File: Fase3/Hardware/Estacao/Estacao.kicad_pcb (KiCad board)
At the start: 2 copper layers, 104.1 x 97.8 mm, 33 parts, among them J1 WCM, J2 I2C-1, J3 I2C-2, J4 I2C-3, J5 GPS, J6 Photo Cel, SW1 SW_Wuerth_450301014042, SW2 SW_Wuerth_450301014042, SW3 SW_Wuerth_450301014042, SW4 Config, SW5 Reset

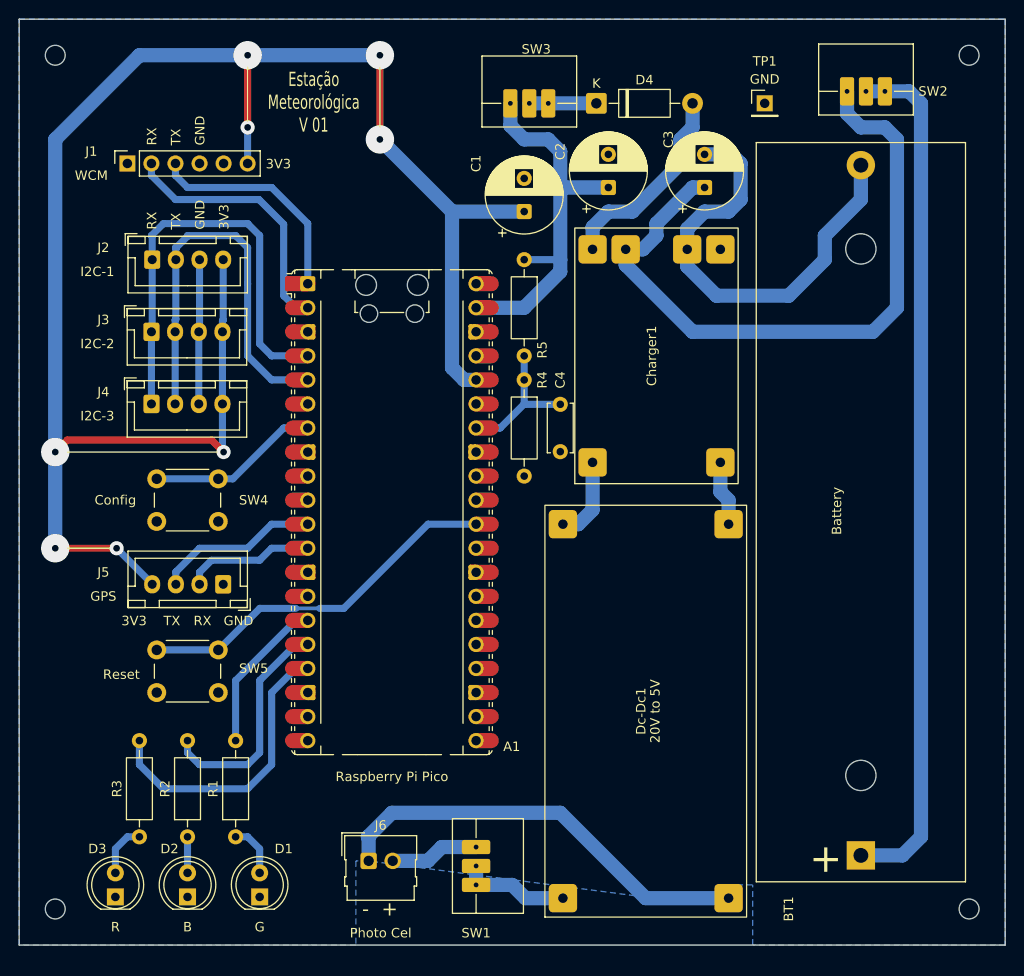
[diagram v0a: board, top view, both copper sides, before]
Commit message: Update PCB V03
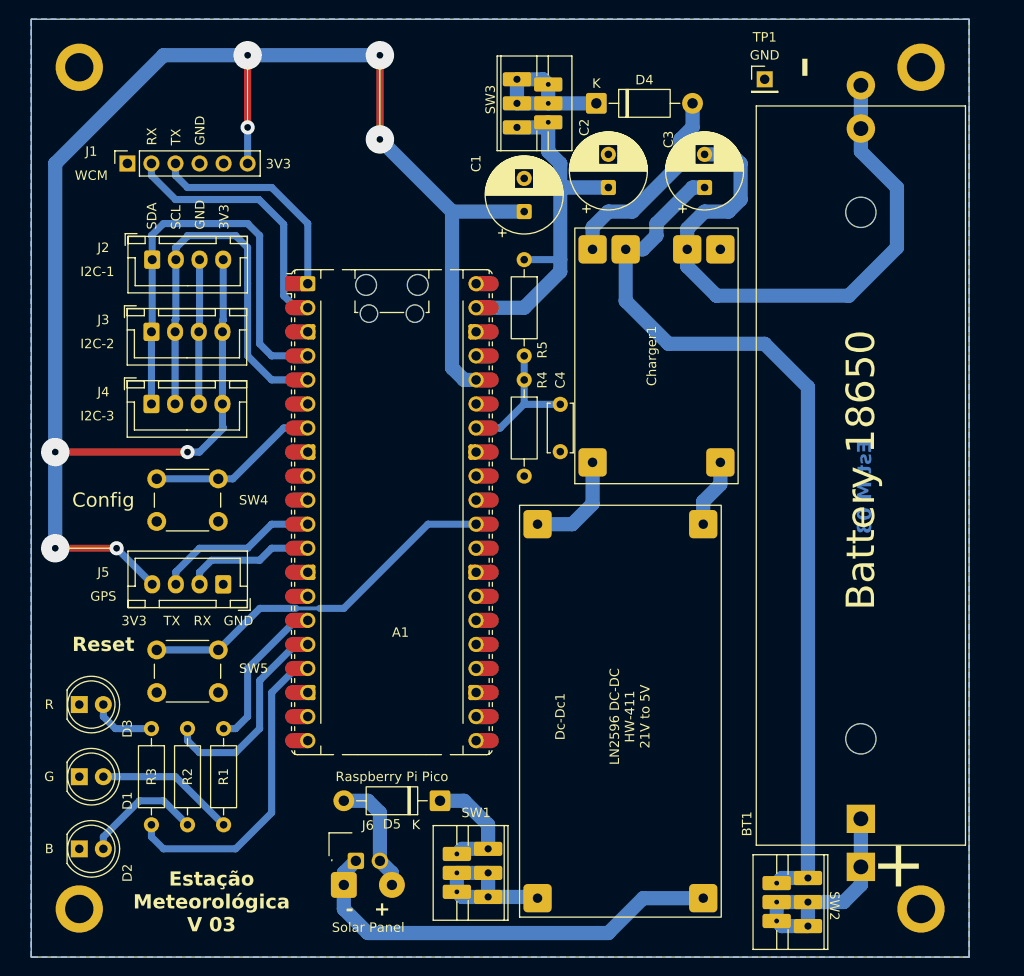
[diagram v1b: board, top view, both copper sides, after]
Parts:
- removed the ? at (194.3, 128.3)
- removed REF** (x3): MountingHole_2.1mm, MountingHole:MountingHole_2.1mm
- added ?: , , F.Cu at (189.2, 39.4)
- added ?: , , F.Cu at (100.3, 39.4)
- added ?: , , F.Cu at (100.3, 128.3)
- added ?: , , F.Cu at (189.2, 128.3)
- added D5: 1N5819, Diode_THT:D_DO-41_SOD81_P10.16mm_Horizontal, F.Cu at (138.4, 116.8)
- BT1: value Battery -> Battery 18650 2000mAh; footprint Battery:BatteryHolder_MPD_BK-18650-PC2 -> PcbLibrary:BatteryHolder_MPD_BK-18650-PC2b
- C3: value C_Polarized -> 100 uF
- C4: value C -> 100n
- Charger1: value ~ -> HW-107
- Dc-Dc1: value 20V to 5V -> LN2596 DC-DC HW-411 21V to 5V
- J6: footprint Connector_Molex:Molex_SL_171971-0002_1x02_P2.54mm_Vertical -> PcbLibrary:Molex_SL_171971-0002_1x02_P2.54mm_Vertical_b
- R1, R2, R3: value R -> 1k
- R4, R5: value R -> 100k
- SW1, SW2, SW3: value SW_Wuerth_450301014042 -> SW_SPDT; footprint PcbLibrary:switch_3p_2mm -> PcbLibrary:switch_3p_2mm_e_2.54mm
- moved SW2 85.8 mm to (177.3, 127.5), turned to -90 degrees
- moved D1 22.9 mm to (100.3, 114.3), turned to 0 degrees
- moved D3 20.7 mm to (100.3, 106.7), turned to 0 degrees
- moved D2 12.5 mm to (100.3, 121.9), turned to 0 degrees
- moved R3 11.5 mm to (108.0, 109.2), turned to -90 degrees
- moved BT1 3.86 mm to (182.9, 118.7)
- moved Dc-Dc1 2.68 mm to (157.5, 107.4)
- moved TP1 2.54 mm to (172.7, 40.6)
- moved R1 1.80 mm to (115.6, 119.4)
- moved SW1 1.46 mm to (143.5, 124.5)
- moved J6 1.35 mm to (129.5, 123.2)
- moved SW3 1.30 mm to (146.6, 43.2), turned to 90 degrees
- moved R2 1.27 mm to (111.8, 119.4)
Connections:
- A1 pad 33: unconnected-(A1-AGND-Pad33) -> GND
- J6 pad 2: Net-(J6-Pin_2) -> Net-(D5-A)
- SW1 pad 1: Net-(Dc-Dc1-IN+) -> Net-(D5-K)
- SW1 pad 3: Net-(J6-Pin_2) -> Net-(Dc-Dc1-IN+)
- SW2 pad 1: Net-(BT1-+) -> Net-(Charger1-Bat+)
- SW2 pad 3: Net-(Charger1-Bat+) -> Net-(BT1-+)
- SW3 pad 1: Net-(D4-K) -> Net-(A1-VSYS)
- SW3 pad 3: Net-(A1-VSYS) -> Net-(D4-K)
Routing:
- net Net-(BT1-+): track 91.0 -> 24.7 mm
- net Net-(Charger1-Bat+): track 72.6 -> 95.6 mm
- net Net-(BT1--): track 47.9 -> 63.2 mm
- net Net-(D5-A): track 0.00 -> 12.5 mm
- net Net-(D5-K): track 0.00 -> 12.2 mm
- net Net-(J6-Pin_2): track 9.41 -> 0.00 mm
- net Net-(D4-K): track 7.08 -> 16.4 mm
- net Net-(D1-A): track 5.61 -> 14.8 mm
- net Net-(D2-A): track 3.81 -> 12.8 mm
- net Net-(Dc-Dc1-IN+): track 11.7 -> 16.6 mm
- net Net-(A1-3V3): track 190.5 -> 186.5 mm
- net Net-(A1-GPIO13): track 31.1 -> 33.6 mm
- net Net-(Charger1-IN+): track 8.78 -> 11.1 mm
- net Net-(A1-GPIO12): track 24.2 -> 22.2 mm
- net Net-(A1-VSYS): track 40.8 -> 39.2 mm
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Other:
- board size 104.1 x 97.8 mm -> 99.1 x 99.1 mm
- board text added: "Est M 03"
- board text added: "Estação Meteorológica V 03"
- board text added: "SCL"
- board text added: "SDA"
- board text added: "Solar Panel"
- board text removed: "Estação Meteorológica V 01"
